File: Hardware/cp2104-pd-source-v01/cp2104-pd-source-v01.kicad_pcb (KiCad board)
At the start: 2 copper layers, 25.4 x 25.4 mm, 1 part, among them U1 LDR6023C

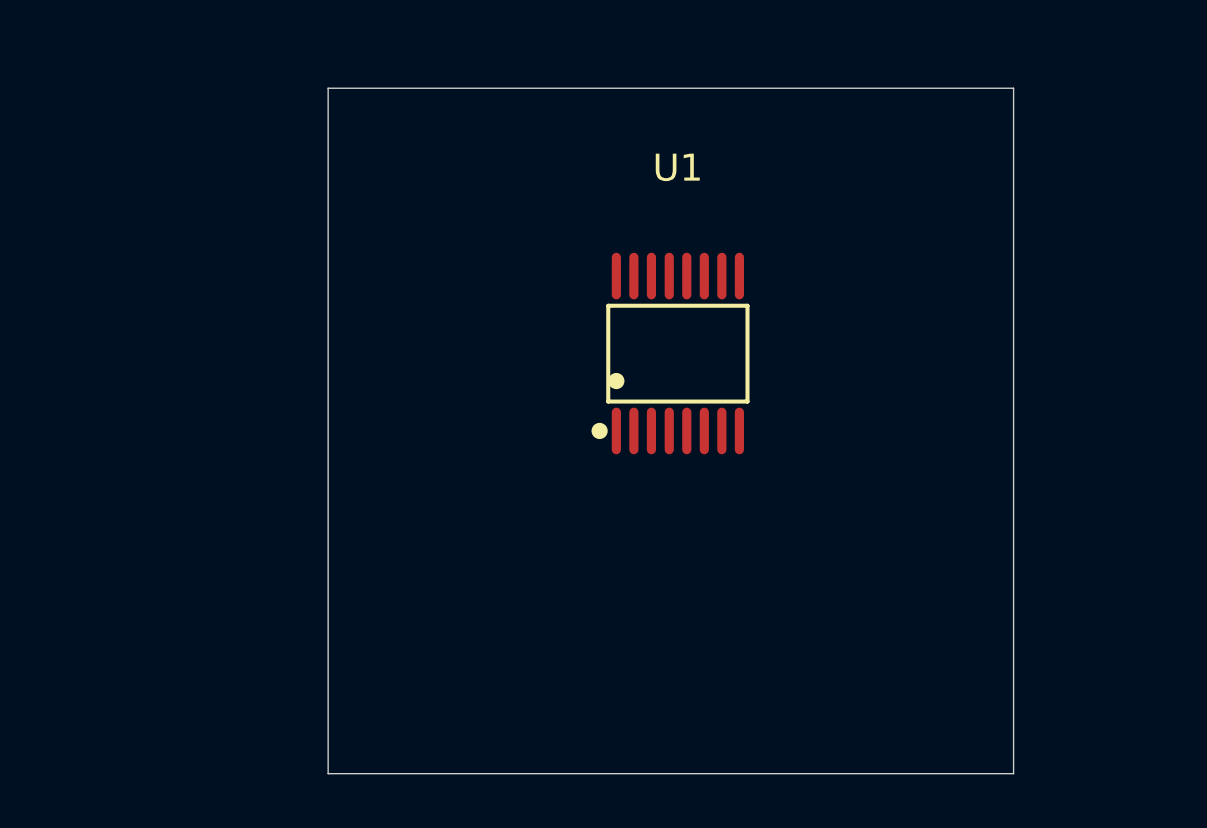
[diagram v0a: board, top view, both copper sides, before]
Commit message: add final pcb
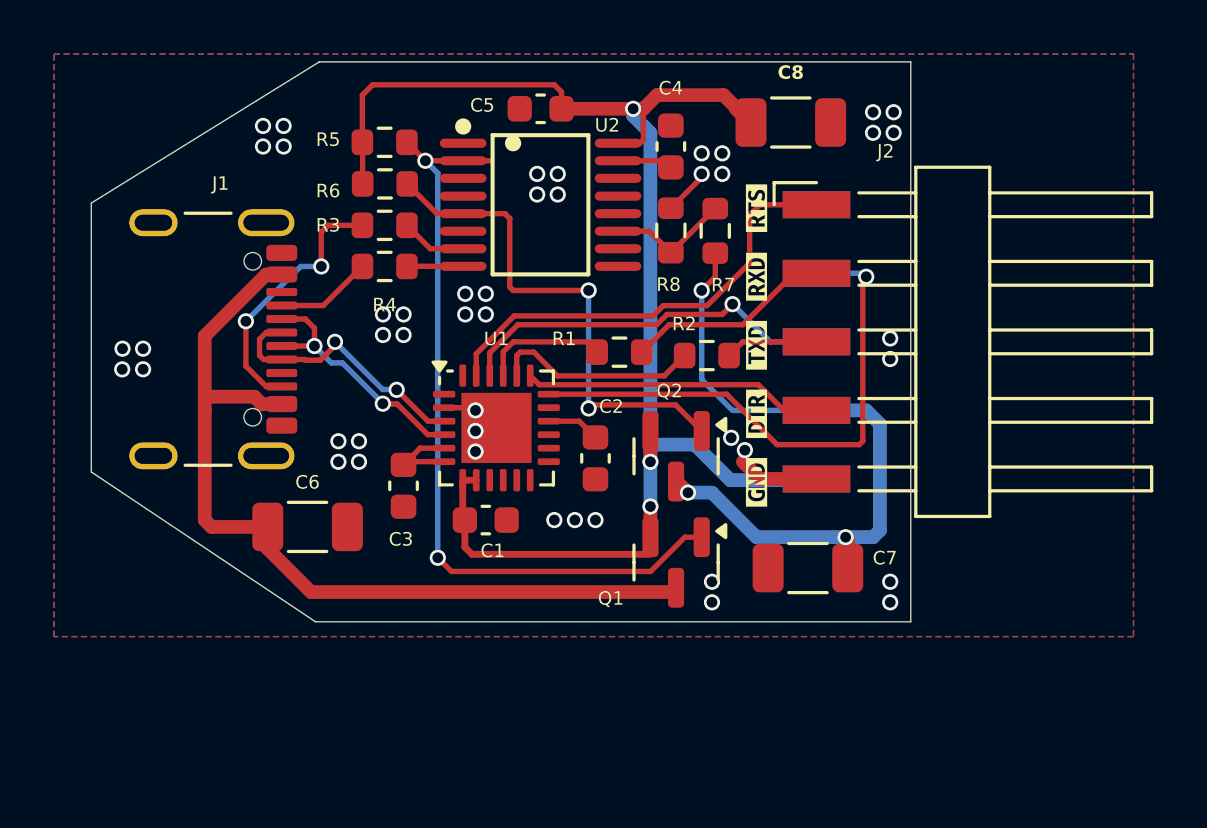
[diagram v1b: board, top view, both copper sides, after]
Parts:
- added C1: 1uF, Capacitor_SMD:C_0603_1608Metric, F.Cu at (132.8, 66.8)
- added C2: 4.7uF, Capacitor_SMD:C_0603_1608Metric, F.Cu at (136.9, 64.5)
- added C3: 1uF, Capacitor_SMD:C_0603_1608Metric, F.Cu at (129.8, 65.5)
- added C4: 1nF, Capacitor_SMD:C_0603_1608Metric, F.Cu at (139.7, 53.0)
- added C5: 100nF, Capacitor_SMD:C_0603_1608Metric, F.Cu at (134.9, 51.6)
- added C6: 22uF, Capacitor_SMD:C_1206_3216Metric, F.Cu at (126.2, 67.1)
- added C7: 22uF, Capacitor_SMD:C_1206_3216Metric, F.Cu at (144.8, 68.6)
- added C8: 22uF, Capacitor_SMD:C_1206_3216Metric, F.Cu at (144.1, 52.1)
- added J1: USB_C_Receptacle_USB2.0_16P, Connector_USB:USB_C_Receptacle_GCT_USB4105-xx-A_16P_TopMnt_Horizontal, F.Cu at (121.6, 60.1)
- added J2: HEADER TOP, Connector_Harwin:Harwin_M20-89005xx_1x05_P2.54mm_Horizontal, F.Cu at (150.6, 60.2)
- added J4: HEADER BOT, Connector_Harwin:Harwin_M20-89005xx_1x05_P2.54mm_Horizontal, B.Cu at (150.6, 60.2)
- added Q1: AO3400A, Package_TO_SOT_SMD:SOT-23, F.Cu at (139.9, 68.4)
- added Q2: AO3400A, Package_TO_SOT_SMD:SOT-23, F.Cu at (139.9, 64.4)
- added R1: 470, Resistor_SMD:R_0603_1608Metric, F.Cu at (137.8, 60.6)
- added R2: 470, Resistor_SMD:R_0603_1608Metric, F.Cu at (141.0, 60.7)
- added R3: 100, Resistor_SMD:R_0603_1608Metric, F.Cu at (129.1, 55.9)
- added R4: 100, Resistor_SMD:R_0603_1608Metric, F.Cu at (129.1, 57.4)
- added R5: 10K, Resistor_SMD:R_0603_1608Metric, F.Cu at (129.1, 52.8)
- added R6: 10K, Resistor_SMD:R_0603_1608Metric, F.Cu at (129.1, 54.3)
- added R7: 36K, Resistor_SMD:R_0603_1608Metric, F.Cu at (141.3, 56.1)
- added R8: 12K, Resistor_SMD:R_0603_1608Metric, F.Cu at (139.7, 56.1)
- added U2: LDR6023C, easyeda2kicad:SSOP-16_L5.0-W4.4-P0.65-LS6.4-BL, F.Cu at (134.9, 55.1)
- added kibuzzard-66B1E901: G***, kibuzzard-66B1E901, F.Cu at (142.9, 60.3)
- added kibuzzard-66B1E90B: G***, kibuzzard-66B1E90B, F.Cu at (142.9, 57.8)
- added kibuzzard-66B1E91A: G***, kibuzzard-66B1E91A, F.Cu at (142.9, 55.2)
- added kibuzzard-66B1E950: G***, kibuzzard-66B1E950, F.Cu at (142.9, 65.4)
- added kibuzzard-66B1E950: G***, kibuzzard-66B1E950, B.Cu at (142.9, 65.4)
- added kibuzzard-66B1E959: G***, kibuzzard-66B1E959, F.Cu at (142.9, 62.9)
- added kibuzzard-66B1E998: G***, kibuzzard-66B1E998, B.Cu at (142.9, 62.9)
- added kibuzzard-66B1E9B1: G***, kibuzzard-66B1E9B1, B.Cu at (142.9, 60.3)
- added kibuzzard-66B1E9B7: G***, kibuzzard-66B1E9B7, B.Cu at (142.9, 57.8)
- added kibuzzard-66B1E9BE: G***, kibuzzard-66B1E9BE, B.Cu at (142.9, 55.2)
- U1: value LDR6023C -> CP2104; footprint easyeda2kicad:SSOP-16_L5.0-W4.4-P0.65-LS6.4-BL -> Package_DFN_QFN:QFN-24-1EP_4x4mm_P0.5mm_EP2.6x2.6mm
- moved U1 7.27 mm to (133.2, 63.4)
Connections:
- U1 pad 16: unconnected-(U1-VDD-Pad16) -> Net-(U1-VPP)
- U1 pad 2: unconnected-(U1-VBEN-Pad2) -> GND
- U1 pad 3: unconnected-(U1-AnaDet-Pad3) -> D+
- U1 pad 4: unconnected-(U1-Vlimited-Pad4) -> D-
- U1 pad 5: unconnected-(U1-VadpEN-Pad5) -> Net-(U1-VDD)
- U1 pad 6: unconnected-(U1-ResetOut-Pad6) -> Net-(U1-VDD)
- U1 pad 7: unconnected-(U1-C0CC2-Pad7) -> +5V
- U1 pad 8: unconnected-(U1-C0CC1-Pad8) -> +5V
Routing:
- net +5V: track 0.00 -> 55.8 mm, vias 0 -> 3
- net VBUS: track 0.00 -> 32.7 mm
- net VBUS_EN: track 0.00 -> 28.8 mm, vias 0 -> 2
- net +5V_IN: track 0.00 -> 25.8 mm, vias 0 -> 3
- net CTS: track 0.00 -> 20.5 mm, vias 0 -> 1
- net VADP_EN: track 0.00 -> 18.9 mm, vias 0 -> 2
- net RTS: track 0.00 -> 16.7 mm
- net DSR: track 0.00 -> 14.3 mm, vias 0 -> 1
- net DTR: track 0.00 -> 11.1 mm
- net D+: track 0.00 -> 10.0 mm, vias 0 -> 2
- net CC2: track 0.00 -> 9.84 mm, vias 0 -> 2
- net D-: track 0.00 -> 9.55 mm, vias 0 -> 2
- net Net-(U1-RXD): track 0.00 -> 7.70 mm
- net RXD0: track 0.00 -> 7.69 mm
- net GND: track 0.00 -> 5.67 mm, vias 0 -> 46
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- added copper zone on B.Cu, net GND
- added copper zone on F.Cu, net GND
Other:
- board size 25.4 x 25.4 mm -> 30.4 x 20.7 mm
